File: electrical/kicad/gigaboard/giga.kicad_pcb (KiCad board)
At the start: 2 copper layers, 88.3 x 54 mm, 2 parts

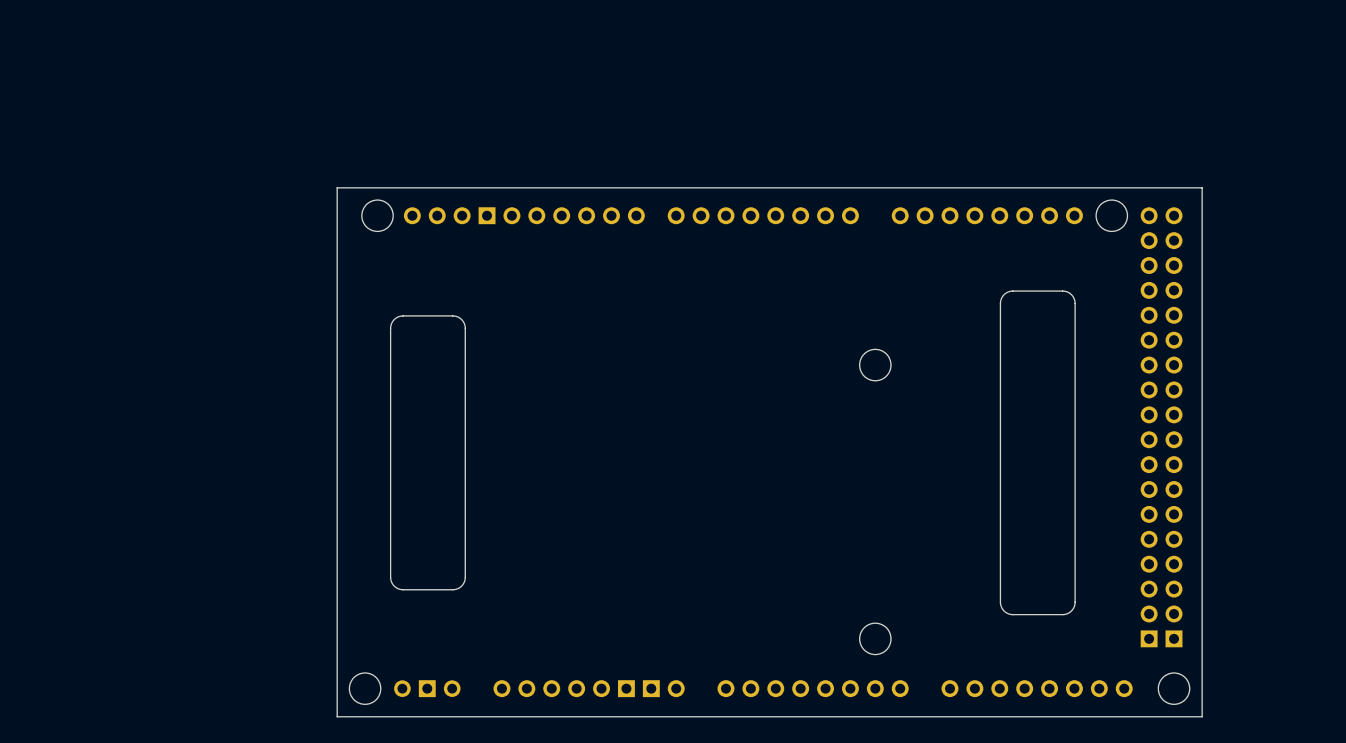
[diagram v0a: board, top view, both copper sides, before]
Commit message: update(giga): pcb layout #01
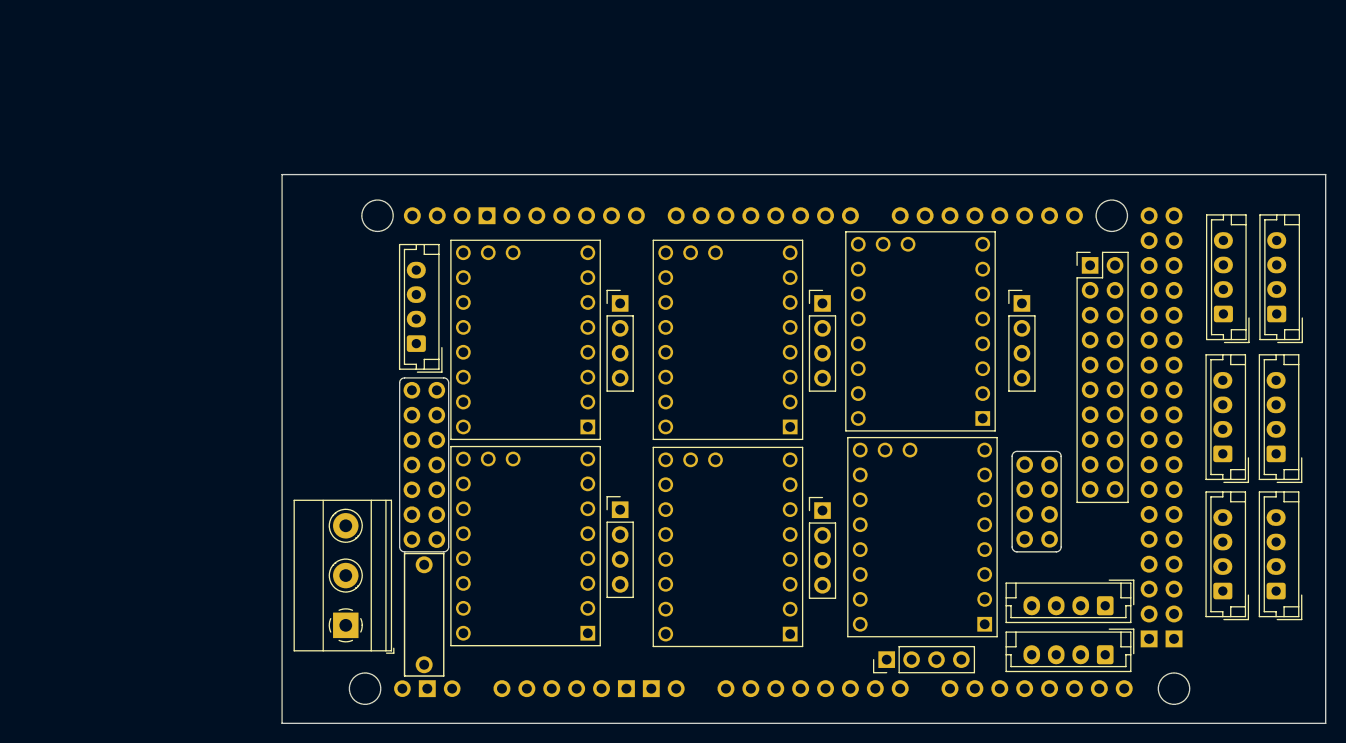
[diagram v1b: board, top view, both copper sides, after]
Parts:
- removed ?: , clipboard:050be39d-fed9-491a-89e1-a26c1a1eb318
- added F1: F_Small, Fuse_TE5_Littlefuse-395Series, F.Cu at (120.0, 89.9)
- added REF**: PinHeader_1x04_P2.54mm_Vertical, Connector_PinHeader_2.54mm:PinHeader_1x04_P2.54mm_Vertical, F.Cu at (181.0, 58.1)
- added REF**: MKS_TMC2209, Motor_Driver:MKS_TMC2209, F.Cu at (151.0, 61.9)
- added REF**: JST_EH_B4B-EH-A_1x04_P2.50mm_Vertical, Connector_JST:JST_EH_B4B-EH-A_1x04_P2.50mm_Vertical, F.Cu at (207.0, 59.2)
- added REF**: TerminalBlock_Phoenix_MKDS-1,5-3-5.08_1x03_P5.08mm_Horizont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, TerminalBlock_Phoenix:TerminalBlock_Phoenix_MKDS-1,5-3-5.08_1x03_P5.08mm_Horizontal, F.Cu at (112.0, 91.0)
- added REF**: MKS_TMC2209, Motor_Driver:MKS_TMC2209, F.Cu at (170.7, 61.0)
- added REF**: MKS_TMC2209, Motor_Driver:MKS_TMC2209, F.Cu at (151.0, 83.0)
- added REF**: PinHeader_1x04_P2.54mm_Vertical, Connector_PinHeader_2.54mm:PinHeader_1x04_P2.54mm_Vertical, F.Cu at (140.0, 58.1)
- added REF**: PinHeader_2x10_P2.54mm_Vertical, Connector_PinHeader_2.54mm:PinHeader_2x10_P2.54mm_Vertical, F.Cu at (188.0, 54.3)
- added REF**: PinHeader_1x04_P2.54mm_Vertical, Connector_PinHeader_2.54mm:PinHeader_1x04_P2.54mm_Vertical, F.Cu at (140.0, 79.2)
- added REF**: JST_EH_B4B-EH-A_1x04_P2.50mm_Vertical, Connector_JST:JST_EH_B4B-EH-A_1x04_P2.50mm_Vertical, F.Cu at (189.5, 89.0)
- added REF**: JST_EH_B4B-EH-A_1x04_P2.50mm_Vertical, Connector_JST:JST_EH_B4B-EH-A_1x04_P2.50mm_Vertical, F.Cu at (201.5, 87.5)
- added REF**: MKS_TMC2209, Motor_Driver:MKS_TMC2209, F.Cu at (130.3, 82.9)
- added REF**: JST_EH_B4B-EH-A_1x04_P2.50mm_Vertical, Connector_JST:JST_EH_B4B-EH-A_1x04_P2.50mm_Vertical, F.Cu at (119.2, 62.2)
- added REF**: JST_EH_B4B-EH-A_1x04_P2.50mm_Vertical, Connector_JST:JST_EH_B4B-EH-A_1x04_P2.50mm_Vertical, F.Cu at (189.5, 94.0)
- added REF**: PinHeader_1x04_P2.54mm_Vertical, Connector_PinHeader_2.54mm:PinHeader_1x04_P2.54mm_Vertical, F.Cu at (160.7, 58.1)
- added REF**: MKS_TMC2209, Motor_Driver:MKS_TMC2209, F.Cu at (170.8, 82.0)
- added REF**: PinHeader_1x04_P2.54mm_Vertical, Connector_PinHeader_2.54mm:PinHeader_1x04_P2.54mm_Vertical, F.Cu at (160.7, 79.3)
- added REF**: JST_EH_B4B-EH-A_1x04_P2.50mm_Vertical, Connector_JST:JST_EH_B4B-EH-A_1x04_P2.50mm_Vertical, F.Cu at (206.9, 73.5)
- added REF**: JST_EH_B4B-EH-A_1x04_P2.50mm_Vertical, Connector_JST:JST_EH_B4B-EH-A_1x04_P2.50mm_Vertical, F.Cu at (206.9, 87.5)
- added REF**: JST_EH_B4B-EH-A_1x04_P2.50mm_Vertical, Connector_JST:JST_EH_B4B-EH-A_1x04_P2.50mm_Vertical, F.Cu at (201.5, 73.5)
- added REF**: MKS_TMC2209, Motor_Driver:MKS_TMC2209, F.Cu at (130.3, 61.9)
- added REF**: JST_EH_B4B-EH-A_1x04_P2.50mm_Vertical, Connector_JST:JST_EH_B4B-EH-A_1x04_P2.50mm_Vertical, F.Cu at (201.6, 59.2)
- added REF**: PinHeader_1x04_P2.54mm_Vertical, Connector_PinHeader_2.54mm:PinHeader_1x04_P2.54mm_Vertical, F.Cu at (167.2, 94.5)
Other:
- board size 88.3 x 54 mm -> 106.5 x 56 mm

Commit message: update(giga): pcb layout #02
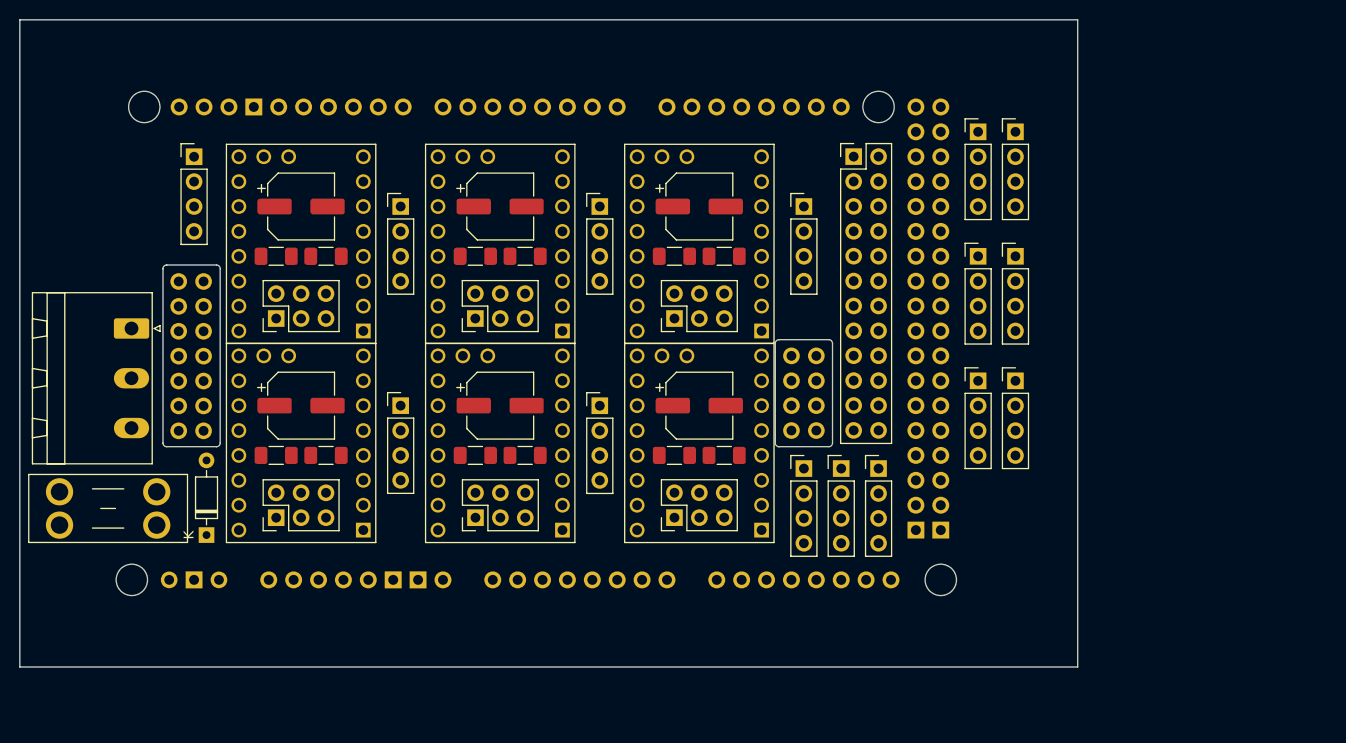
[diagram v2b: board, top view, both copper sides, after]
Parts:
- removed REF** (x6): PinHeader_1x04_P2.54mm_Vertical, Connector_PinHeader_2.54mm:PinHeader_1x04_P2.54mm_Vertical
- removed REF** (x6): MKS_TMC2209, Motor_Driver:MKS_TMC2209
- removed REF** (x9): JST_EH_B4B-EH-A_1x04_P2.50mm_Vertical, Connector_JST:JST_EH_B4B-EH-A_1x04_P2.50mm_Vertical
- removed REF**: TerminalBlock_Phoenix_MKDS-1,5-3-5.08_1x03_P5.08mm_Horizont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, TerminalBlock_Phoenix:TerminalBlock_Phoenix_MKDS-1,5-3-5.08_1x03_P5.08mm_Horizontal
- removed REF**: PinHeader_2x10_P2.54mm_Vertical, Connector_PinHeader_2.54mm:PinHeader_2x10_P2.54mm_Vertical
- added C1: 100uF, Capacitor_SMD:CP_Elec_6.3x7.7, F.Cu at (107.4, 48.3)
- added C2: 100uF, Capacitor_SMD:CP_Elec_6.3x7.7, F.Cu at (107.4, 68.6)
- added C3: 100uF, Capacitor_SMD:CP_Elec_6.3x7.7, F.Cu at (127.8, 48.3)
- added C4: 100uF, Capacitor_SMD:CP_Elec_6.3x7.7, F.Cu at (127.8, 68.6)
- added C5: 100uF, Capacitor_SMD:CP_Elec_6.3x7.7, F.Cu at (148.1, 48.3)
- added C6: 100uF, Capacitor_SMD:CP_Elec_6.3x7.7, F.Cu at (148.1, 68.6)
- added D1: D, Diode_THT:D_DO-35_SOD27_P7.62mm_Horizontal, F.Cu at (97.8, 81.8)
- added J1: Conn_02x03_Counter_Clockwise, Connector_PinHeader_2.54mm:PinHeader_2x03_P2.54mm_Vertical, F.Cu at (104.9, 59.7)
- added J10: Conn_01x04, Connector_PinHeader_2.54mm:PinHeader_1x04_P2.54mm_Vertical, F.Cu at (137.9, 68.6)
- added J11: Conn_01x04, Connector_PinHeader_2.54mm:PinHeader_1x04_P2.54mm_Vertical, F.Cu at (158.8, 48.3)
- added J12: Conn_01x04, Connector_PinHeader_2.54mm:PinHeader_1x04_P2.54mm_Vertical, F.Cu at (158.8, 75.0)
- added J13: Conn_01x04, Connector_PinHeader_2.54mm:PinHeader_1x04_P2.54mm_Vertical, F.Cu at (176.5, 40.6)
- added J14: Conn_01x04, Connector_PinHeader_2.54mm:PinHeader_1x04_P2.54mm_Vertical, F.Cu at (176.5, 53.3)
- added J15: Conn_01x04, Connector_PinHeader_2.54mm:PinHeader_1x04_P2.54mm_Vertical, F.Cu at (176.5, 66.0)
- added J16: Conn_01x04, Connector_PinHeader_2.54mm:PinHeader_1x04_P2.54mm_Vertical, F.Cu at (180.3, 40.6)
- added J17: Conn_01x04, Connector_PinHeader_2.54mm:PinHeader_1x04_P2.54mm_Vertical, F.Cu at (180.3, 53.3)
- added J18: Conn_01x04, Connector_PinHeader_2.54mm:PinHeader_1x04_P2.54mm_Vertical, F.Cu at (180.3, 66.0)
- added J19: Conn_01x04, Connector_PinHeader_2.54mm:PinHeader_1x04_P2.54mm_Vertical, F.Cu at (96.5, 43.2)
- added J2: Conn_02x04_Counter_Clockwise, Connector_PinHeader_2.54mm:PinHeader_2x03_P2.54mm_Vertical, F.Cu at (104.9, 80.0)
- added J20: Conn_01x04, Connector_PinHeader_2.54mm:PinHeader_1x04_P2.54mm_Vertical, F.Cu at (162.6, 75.0)
- added J21: Conn_01x04, Connector_PinHeader_2.54mm:PinHeader_1x04_P2.54mm_Vertical, F.Cu at (166.4, 75.0)
- added J22: Screw_Terminal_01x03, Connector_Phoenix_MSTB:PhoenixContact_MSTBA_2,5_3-G-5,08_1x03_P5.08mm_Horizontal, F.Cu at (90.1, 60.7)
- added J23: Conn_02x12_Counter_Clockwise, Connector_PinHeader_2.54mm:PinHeader_2x12_P2.54mm_Vertical, F.Cu at (163.8, 43.2)
- added J3: Conn_02x04_Counter_Clockwise, Connector_PinHeader_2.54mm:PinHeader_2x03_P2.54mm_Vertical, F.Cu at (125.2, 59.7)
- added J4: Conn_02x04_Counter_Clockwise, Connector_PinHeader_2.54mm:PinHeader_2x03_P2.54mm_Vertical, F.Cu at (125.2, 80.0)
- added J5: Conn_02x04_Counter_Clockwise, Connector_PinHeader_2.54mm:PinHeader_2x03_P2.54mm_Vertical, F.Cu at (145.5, 59.7)
- added J6: Conn_02x04_Counter_Clockwise, Connector_PinHeader_2.54mm:PinHeader_2x03_P2.54mm_Vertical, F.Cu at (145.5, 80.0)
- added J7: Conn_01x04, Connector_PinHeader_2.54mm:PinHeader_1x04_P2.54mm_Vertical, F.Cu at (117.6, 48.3)
- added J8: Conn_01x04, Connector_PinHeader_2.54mm:PinHeader_1x04_P2.54mm_Vertical, F.Cu at (117.6, 68.6)
- added J9: Conn_01x04, Connector_PinHeader_2.54mm:PinHeader_1x04_P2.54mm_Vertical, F.Cu at (137.9, 48.3)
- added R1: 100k, Resistor_SMD:R_1206_3216Metric_Pad1.30x1.75mm_HandSolder, F.Cu at (104.9, 53.3)
- added R10: 10k, Resistor_SMD:R_1206_3216Metric_Pad1.30x1.75mm_HandSolder, F.Cu at (130.3, 73.7)
- added R11: 10k, Resistor_SMD:R_1206_3216Metric_Pad1.30x1.75mm_HandSolder, F.Cu at (150.6, 53.3)
- added R12: 10k, Resistor_SMD:R_1206_3216Metric_Pad1.30x1.75mm_HandSolder, F.Cu at (150.6, 73.7)
- added R2: 100k, Resistor_SMD:R_1206_3216Metric_Pad1.30x1.75mm_HandSolder, F.Cu at (104.9, 73.7)
- added R3: 100k, Resistor_SMD:R_1206_3216Metric_Pad1.30x1.75mm_HandSolder, F.Cu at (125.2, 53.3)
- added R4: 100k, Resistor_SMD:R_1206_3216Metric_Pad1.30x1.75mm_HandSolder, F.Cu at (125.2, 73.7)
- added R5: 100k, Resistor_SMD:R_1206_3216Metric_Pad1.30x1.75mm_HandSolder, F.Cu at (145.5, 53.3)
- added R6: 100k, Resistor_SMD:R_1206_3216Metric_Pad1.30x1.75mm_HandSolder, F.Cu at (145.5, 73.7)
- added R7: 10k, Resistor_SMD:R_1206_3216Metric_Pad1.30x1.75mm_HandSolder, F.Cu at (110.0, 53.3)
- added R8: 10k, Resistor_SMD:R_1206_3216Metric_Pad1.30x1.75mm_HandSolder, F.Cu at (110.0, 73.7)
- added R9: 10k, Resistor_SMD:R_1206_3216Metric_Pad1.30x1.75mm_HandSolder, F.Cu at (130.3, 53.3)
- added U1: TMC2209, Motor_Driver:MKS_TMC2209, F.Cu at (107.4, 52.1)
- added U2: TMC2209, Motor_Driver:MKS_TMC2209, F.Cu at (107.4, 72.4)
- added U3: TMC2209, Motor_Driver:MKS_TMC2209, F.Cu at (127.8, 52.1)
- added U4: TMC2209, Motor_Driver:MKS_TMC2209, F.Cu at (127.8, 72.4)
- added U5: TMC2209, Motor_Driver:MKS_TMC2209, F.Cu at (148.1, 52.1)
- added U6: TMC2209, Motor_Driver:MKS_TMC2209, F.Cu at (148.1, 72.4)
- F1: footprint Fuse_TE5_Littlefuse-395Series -> Fuse:Fuseholder_Blade_Mini_Keystone_3568
- moved F1 39.3 mm to (82.8, 77.4), turned to 0 degrees
- moved A1 26.3 mm to (76.2, 88.9)
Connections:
- A1 pad AREF: /BAT_MAX -> /+3.3V
- A1 pad D22: /TCA_RST -> /ESTOP
- A1 pad D54: (no net) -> unconnected-(A1-PadD54)
- A1 pad D55: (no net) -> unconnected-(A1-PadD55)
- A1 pad D56: (no net) -> unconnected-(A1-PadD56)
- A1 pad D57: (no net) -> unconnected-(A1-PadD57)
- A1 pad D58: (no net) -> unconnected-(A1-PadD58)
- A1 pad D59: (no net) -> unconnected-(A1-PadD59)
- A1 pad D60: (no net) -> unconnected-(A1-PadD60)
- A1 pad D61: (no net) -> unconnected-(A1-PadD61)
- A1 pad D62: (no net) -> unconnected-(A1-PadD62)
- A1 pad D63: (no net) -> unconnected-(A1-PadD63)
- A1 pad D64: (no net) -> unconnected-(A1-PadD64)
- A1 pad D65: (no net) -> unconnected-(A1-PadD65)
- A1 pad D66: (no net) -> unconnected-(A1-PadD66)
- A1 pad D67: (no net) -> unconnected-(A1-PadD67)
- A1 pad D68: (no net) -> unconnected-(A1-PadD68)
- A1 pad D69: (no net) -> unconnected-(A1-PadD69)
- A1 pad D70: (no net) -> unconnected-(A1-PadD70)
- A1 pad D71: (no net) -> unconnected-(A1-PadD71)
- A1 pad D72: (no net) -> unconnected-(A1-PadD72)
- A1 pad D73: (no net) -> unconnected-(A1-PadD73)
- A1 pad D74: (no net) -> unconnected-(A1-PadD74)
- A1 pad D75: (no net) -> unconnected-(A1-PadD75)
- F1 pad 1: (no net) -> /VM
- F1 pad 2: (no net) -> Net-(D1-K)
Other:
- board size 106.5 x 56 mm -> 108 x 66 mm
